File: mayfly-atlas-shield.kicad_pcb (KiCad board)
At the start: 2 copper layers, 66 x 94 mm, 36 parts, among them J1 Conn_Coaxial, J2 Conn_Coaxial, J3 Conn_Coaxial, J4 Conn_Coaxial, J5 Conn_02x10_Counter_Clockwise, J6 Conn_02x10_Counter_Clockwise, U1 ISO1540, U2 CRE1S0505SC, U3 ISO1540, U4 CRE1S0505SC, U5 ISO1540, U6 CRE1S0505SC

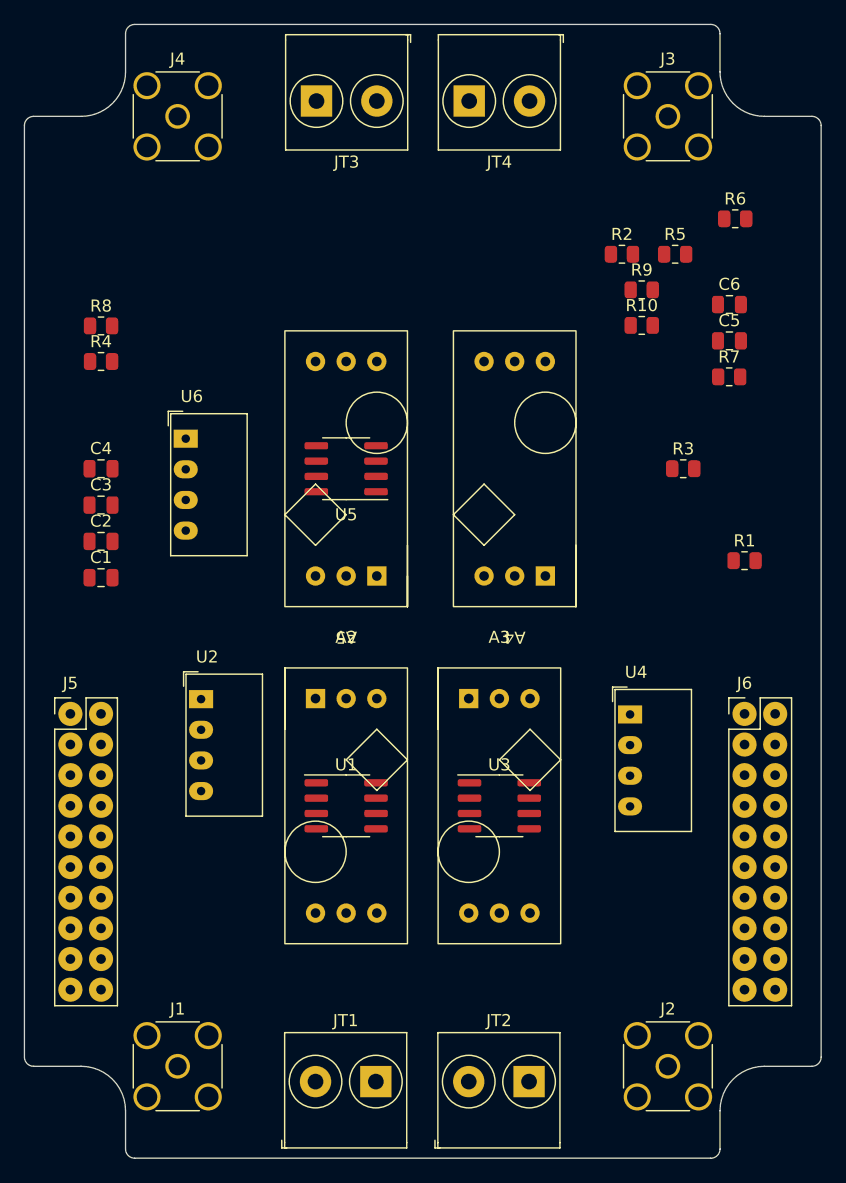
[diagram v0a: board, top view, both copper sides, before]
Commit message: pcb layout
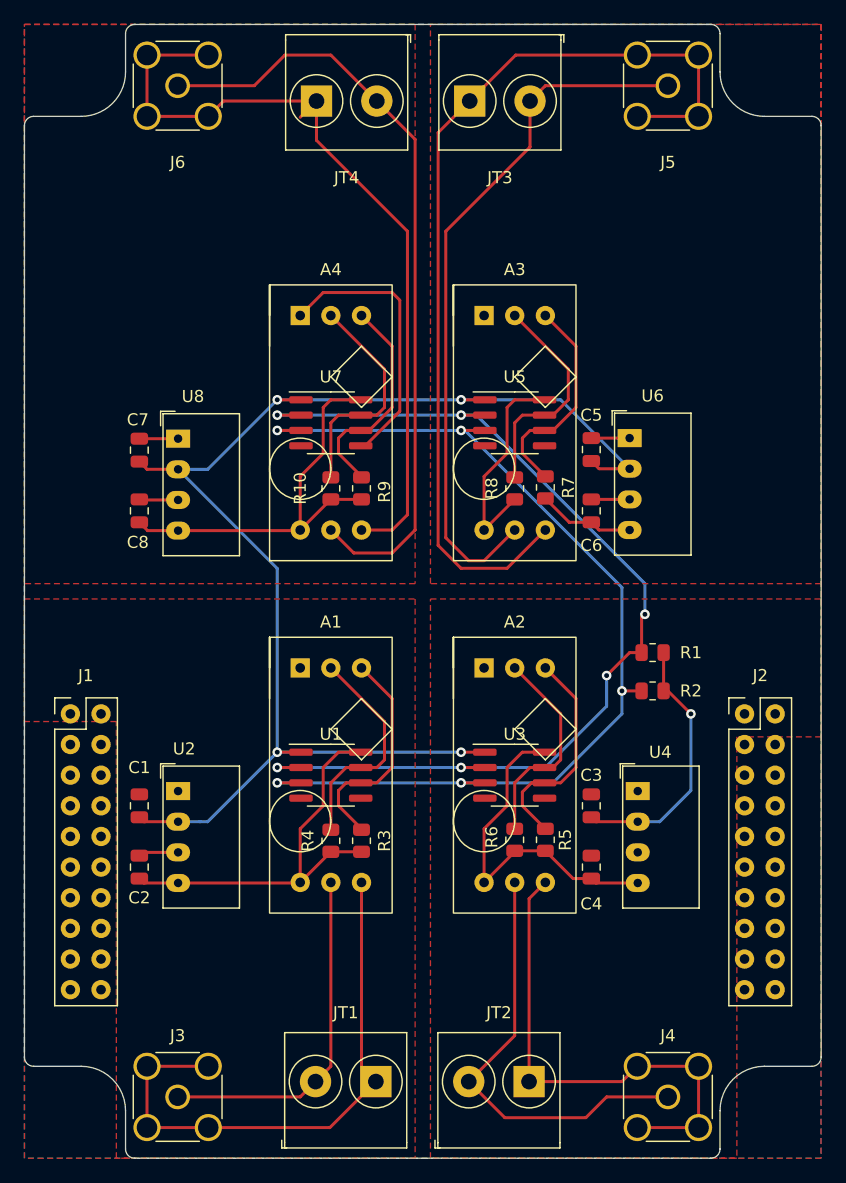
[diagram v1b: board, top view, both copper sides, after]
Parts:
- removed the R5 at (136.5, 88.9)
- removed the R6 at (141.5, 86.0)
- added C7: 4.7u, Capacitor_SMD:C_0805_2012Metric, F.Cu at (92.1, 105.1)
- added C8: 4.7u, Capacitor_SMD:C_0805_2012Metric, F.Cu at (92.1, 110.2)
- added R7: 4.7k, Resistor_SMD:R_0805_2012Metric, F.Cu at (125.7, 108.2)
- added R8: 4.7k, Resistor_SMD:R_0805_2012Metric, F.Cu at (123.2, 108.3)
- added U7: ISO1540, Package_SO:SOIC-8_3.9x4.9mm_P1.27mm, F.Cu at (108.0, 102.9)
- added U8: CRE1S0505SC, Converter_DCDC:Converter_DCDC_Murata_CRE1xxxxxxSC_THT, F.Cu at (95.3, 104.2)
- J1, J2: value Conn_Coaxial -> Conn_02x10_Counter_Clockwise; footprint toolbox-connector:SMA_Vertical -> toolbox-mayfly:Mayfly_v1_Headers
- J5, J6: value Conn_02x10_Counter_Clockwise -> Conn_Coaxial; footprint toolbox-mayfly:Mayfly_v1_Headers -> toolbox-connector:SMA_Vertical
- moved J3 90.9 mm to (95.2, 158.8)
- moved J4 90.9 mm to (135.9, 158.8)
- moved J5 71.9 mm to (135.9, 74.9)
- moved J6 70.1 mm to (95.2, 74.9)
- moved R2 54.8 mm to (134.6, 125.1)
- moved C4 48.8 mm to (129.5, 139.7), turned to 90 degrees
- moved R5 46.3 mm to (125.7, 137.4), turned to -90 degrees
- moved C3 44.8 mm to (129.5, 134.6), turned to -90 degrees
- moved R4 44.1 mm to (108.0, 137.5), turned to -90 degrees
- moved R6 43.9 mm to (123.2, 137.4), turned to -90 degrees
- moved R3 40.8 mm to (110.5, 137.5), turned to -90 degrees
- moved U2 38.0 mm to (95.3, 133.4)
- moved U4 37.0 mm to (133.4, 133.4)
- moved U6 36.8 mm to (132.7, 104.1)
- moved C2 33.2 mm to (92.1, 139.7), turned to 90 degrees
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- renumbered A2 to A1, A3 to A2, A4 to A3, A5 to A4, C3 to C1, C4 to C2, C1 to C3, C2 to C4, R7 to R1, R2 to R10, R8 to R2, R9 to R5, R10 to R6, R1 to R9, U3 to U1, U4 to U2, U1 to U3, U2 to U4
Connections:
- A1 pad 5: Net-(A2-Pad5) -> Net-(A1-Pad5)
- A1 pad 6: Net-(A2-Pad6) -> Net-(A1-Pad6)
- A2 pad 5: Net-(A3-Pad5) -> Net-(A2-Pad5)
- A2 pad 6: Net-(A3-Pad6) -> Net-(A2-Pad6)
- A3 pad 5: Net-(A4-Pad5) -> Net-(A3-Pad5)
- A3 pad 6: Net-(A4-Pad6) -> Net-(A3-Pad6)
- A4 pad 1: /SCL_3 -> /SCL_4
- A4 pad 2: /SDA_3 -> /SDA_4
- A4 pad 3: GND_ISO_3 -> GND_ISO_4
- A4 pad 4: +5V_ISO_3 -> +5V_ISO_4
- A4 pad 5: Net-(A5-Pad5) -> Net-(A4-Pad5)
- A4 pad 6: Net-(A5-Pad6) -> Net-(A4-Pad6)
- C2 pad 1: +5V_ISO_2 -> +5V_ISO_1
- C2 pad 2: GND_ISO_2 -> GND_ISO_1
- C4 pad 1: +5V_ISO_1 -> +5V_ISO_2
- C4 pad 2: GND_ISO_1 -> GND_ISO_2
- J1 pad 1: Net-(A2-Pad5) -> unconnected-(J1-Pad1)
- J1 pad 2: Net-(A2-Pad6) -> unconnected-(J1-Pad2)
- J2 pad 1: Net-(A3-Pad5) -> unconnected-(J2-Pad1)
- J2 pad 2: Net-(A3-Pad6) -> unconnected-(J2-Pad2)
- J3 pad 1: Net-(A4-Pad5) -> Net-(A1-Pad5)
- J3 pad 2: Net-(A4-Pad6) -> Net-(A1-Pad6)
- J4 pad 1: Net-(A5-Pad5) -> Net-(A2-Pad5)
- J4 pad 2: Net-(A5-Pad6) -> Net-(A2-Pad6)
- J5 pad 1: unconnected-(J5-Pad1) -> Net-(A3-Pad5)
- J5 pad 2: unconnected-(J5-Pad2) -> Net-(A3-Pad6)
- J6 pad 1: unconnected-(J6-Pad1) -> Net-(A4-Pad5)
- J6 pad 2: unconnected-(J6-Pad2) -> Net-(A4-Pad6)
- JT1 pad 1: Net-(A2-Pad5) -> Net-(A1-Pad5)
- JT1 pad 2: Net-(A2-Pad6) -> Net-(A1-Pad6)
- JT2 pad 1: Net-(A3-Pad5) -> Net-(A2-Pad5)
- JT2 pad 2: Net-(A3-Pad6) -> Net-(A2-Pad6)
- JT3 pad 1: Net-(A4-Pad5) -> Net-(A3-Pad5)
- JT3 pad 2: Net-(A4-Pad6) -> Net-(A3-Pad6)
- JT4 pad 1: Net-(A5-Pad5) -> Net-(A4-Pad5)
- JT4 pad 2: Net-(A5-Pad6) -> Net-(A4-Pad6)
- R1 pad 1: /SCL_2 -> /SDA
- R1 pad 2: +5V_ISO_2 -> +5V
- R10 pad 1: /SCL -> /SDA_4
- R10 pad 2: +5V -> +5V_ISO_4
- R2 pad 1: /SDA_2 -> /SCL
- R2 pad 2: +5V_ISO_2 -> +5V
- R5 pad 1: /SCL_3 -> /SCL_2
- R5 pad 2: +5V_ISO_3 -> +5V_ISO_2
- R6 pad 1: /SDA_3 -> /SDA_2
- R6 pad 2: +5V_ISO_3 -> +5V_ISO_2
- R9 pad 1: /SDA -> /SCL_4
- R9 pad 2: +5V -> +5V_ISO_4
- U1 pad 5: GND_ISO_2 -> GND_ISO_1
- U1 pad 6: /SCL_2 -> /SCL_1
- U1 pad 7: /SDA_2 -> /SDA_1
- U1 pad 8: +5V_ISO_2 -> +5V_ISO_1
- U2 pad 3: GND_ISO_2 -> GND_ISO_1
- U2 pad 4: +5V_ISO_2 -> +5V_ISO_1
- U3 pad 5: GND_ISO_1 -> GND_ISO_2
- U3 pad 6: /SCL_1 -> /SCL_2
- U3 pad 7: /SDA_1 -> /SDA_2
- U3 pad 8: +5V_ISO_1 -> +5V_ISO_2
- U4 pad 3: GND_ISO_1 -> GND_ISO_2
- U4 pad 4: +5V_ISO_1 -> +5V_ISO_2
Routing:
- net +5V: track 0.00 -> 135.6 mm, vias 0 -> 5
- net /SDA: track 0.00 -> 85.6 mm, vias 0 -> 6
- net /SCL: track 0.00 -> 84.9 mm, vias 0 -> 5
- net Net-(A3-Pad6): track 0.00 -> 79.6 mm
- net Net-(A4-Pad6): track 0.00 -> 68.4 mm
- net Net-(A4-Pad5): track 0.00 -> 64.6 mm
- net Net-(A3-Pad5): track 0.00 -> 58.6 mm
- net Net-(A1-Pad6): track 0.00 -> 47.7 mm
- net Net-(A2-Pad6): track 0.00 -> 41.8 mm
- net Net-(A2-Pad5): track 0.00 -> 36.5 mm
- net +5V_ISO_4: track 0.00 -> 34.1 mm
- net +5V_ISO_1: track 0.00 -> 33.8 mm
- net Net-(A1-Pad5): track 0.00 -> 29.0 mm
- net +5V_ISO_2: track 0.00 -> 28.9 mm
- net GND_ISO_4: track 0.00 -> 26.2 mm
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- added copper zone on B.Cu, net GND
- added copper zone on F.Cu, net GND
- added copper zone on F.Cu, net GND_ISO_1
- added copper zone on F.Cu, net GND_ISO_2
- added copper zone on F.Cu, net GND_ISO_3
- added copper zone on F.Cu, net GND_ISO_4
